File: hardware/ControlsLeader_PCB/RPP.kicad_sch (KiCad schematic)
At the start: 11 parts, among them Q17 NVMFWS1D7N04XMT1G, Q2 NVMFWS1D7N04XMT1G

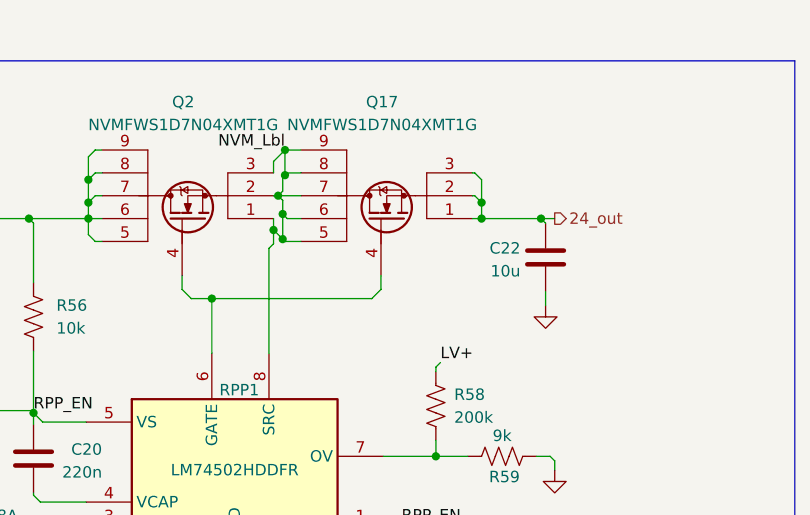
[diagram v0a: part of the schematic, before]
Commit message: Steering Angle Sensor SCH changes
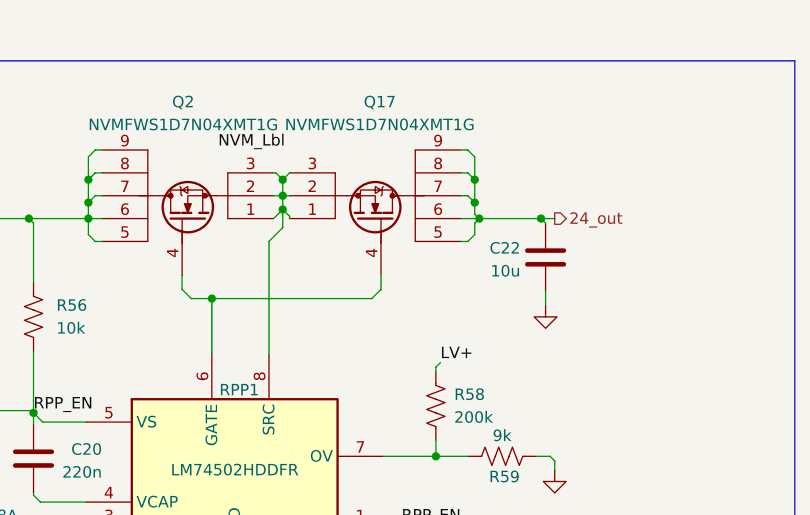
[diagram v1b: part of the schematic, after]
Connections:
- net 24_out: now also Q17.5, Q17.6, Q17.7, Q17.8, Q17.9; no longer Q17.1, Q17.2, Q17.3
- net NVM_Lbl: no longer Q17.5, Q17.6, Q17.7, Q17.8, Q17.9, Q2.1, Q2.2, Q2.3, RPP1.8 (SRC)
- new net: Q17.1, Q17.2, Q17.3, Q2.1, Q2.2, Q2.3, RPP1.8 (SRC)
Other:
- moved on the sheet: Q17
